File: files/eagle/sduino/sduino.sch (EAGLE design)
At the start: 13 parts, among them IC1 ATMEGA48/88/168-AU

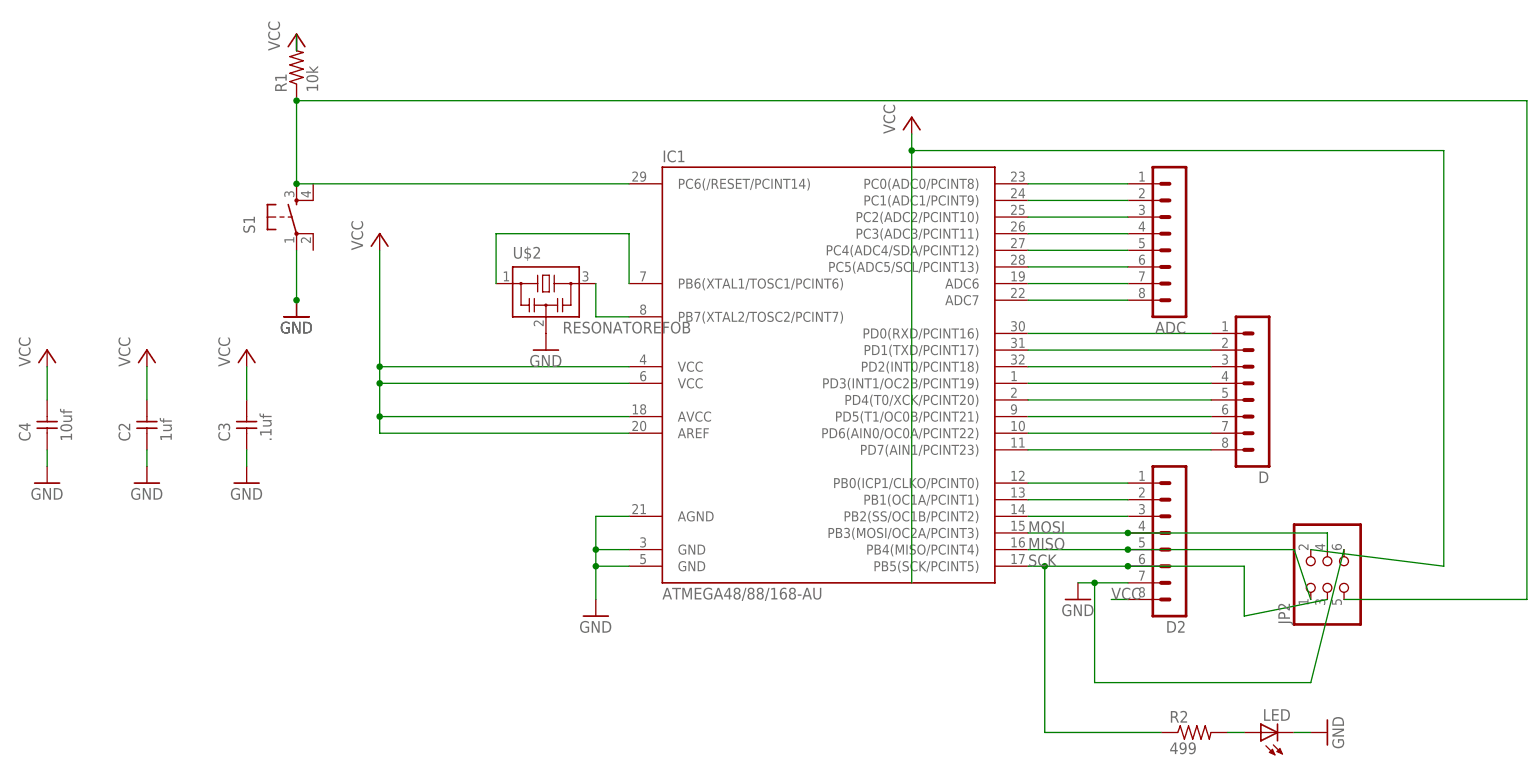
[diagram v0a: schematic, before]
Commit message: typo
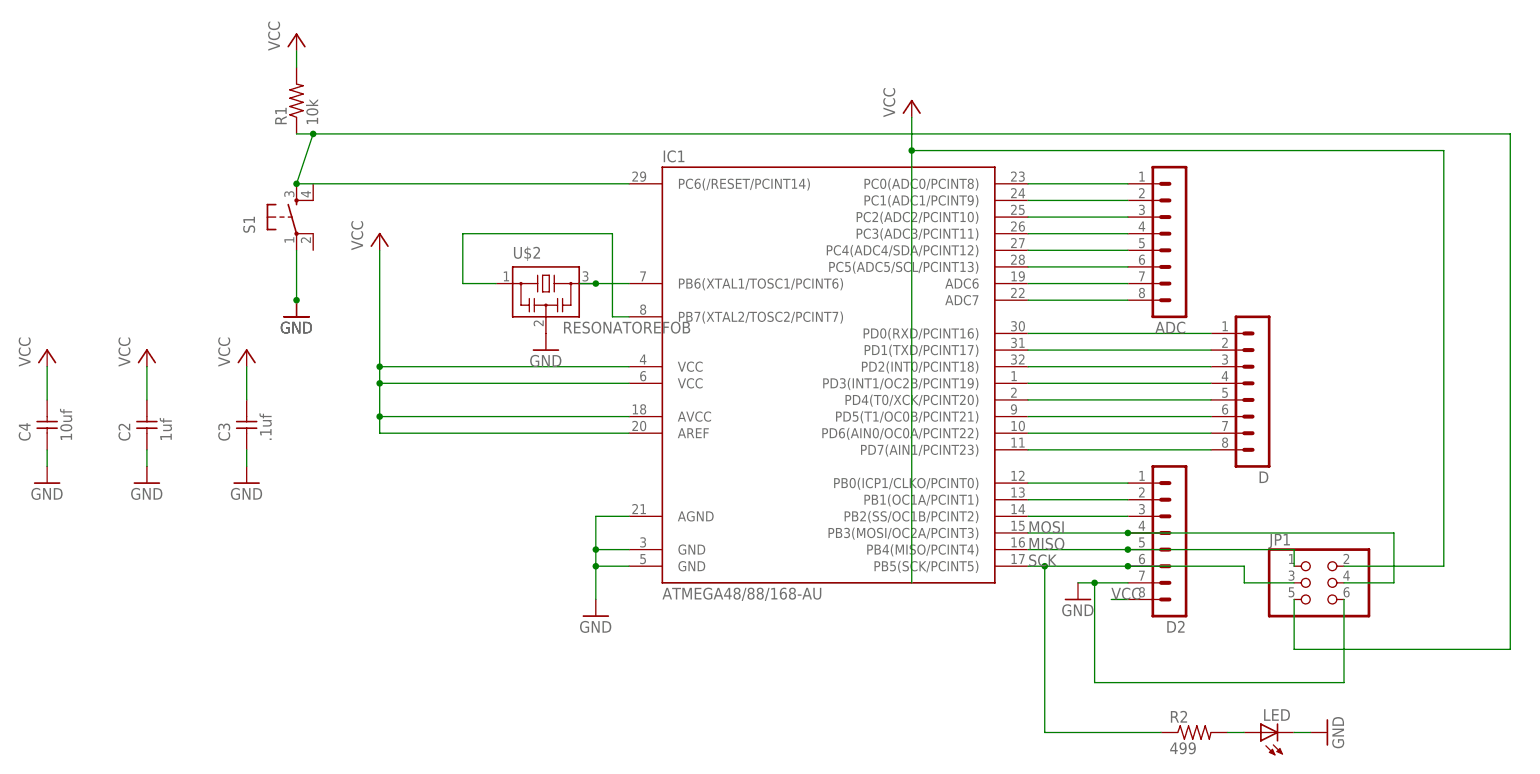
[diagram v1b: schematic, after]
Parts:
- removed JP2: (no value), fab:PINHD-2X3-SMD
- added JP1: (no value), pinhead:PINHD-2X3
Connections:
- removed net N$16: IC1.PB7(XTAL2/TOSC2/PCINT7), U$2.3
- new net N$9: IC1.PB6(XTAL1/TOSC1/PCINT6), U$2.3
- net GND: now also JP1.6; no longer JP2.6
- net MISO: now also JP1.1; no longer JP2.1
- net MOSI: now also JP1.4; no longer JP2.4
- net N$1: now also IC1.PB7(XTAL2/TOSC2/PCINT7); no longer IC1.PB6(XTAL1/TOSC1/PCINT6)
- net RST: now also JP1.5; no longer JP2.5
- net SCK: now also JP1.3; no longer JP2.3
- net VCC: now also JP1.2; no longer JP2.2
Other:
- moved on the sheet: R1
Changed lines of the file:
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@@
 <part name="U$2" library="fab" deviceset="RESONATOR" device="EFOB"/>
 <part name="GND10" library="supply1" deviceset="GND" device=""/>
-<part name="JP2" library="fab" deviceset="PINHD-2X3-SMD" device=""/>
+<part name="JP1" library="pinhead" deviceset="PINHD-2X3" device=""/>
 </parts>
 <sheets>
@@
 <instance part="GND1" gate="1" x="-40.64" y="58.42"/>
 <instance part="GND2" gate="1" x="5.08" y="12.7"/>
-<instance part="R1" gate="G$1" x="-40.64" y="96.52" rot="R90"/>
+<instance part="R1" gate="G$1" x="-40.64" y="91.44" rot="R90"/>
 <instance part="S1" gate="2" x="-40.64" y="73.66"/>
 <instance part="D" gate="1" x="106.68" y="48.26" rot="R180"/>
@@
 <instance part="C4" gate="1" x="-78.74" y="43.18" rot="R90"/>
 <instance part="ADC" gate="1" x="93.98" y="71.12" rot="R180"/>
-<instance part="P+3" gate="VCC" x="53.34" y="88.9"/>
+<instance part="P+3" gate="VCC" x="53.34" y="91.44"/>
 <instance part="D2" gate="1" x="93.98" y="25.4" rot="R180"/>
 <instance part="GND9" gate="1" x="78.74" y="15.24"/>
 <instance part="U$2" gate="G$1" x="-2.54" y="63.5"/>
 <instance part="GND10" gate="1" x="-2.54" y="53.34"/>
-<instance part="JP2" gate="A" x="116.84" y="17.78" rot="R90"/>
+<instance part="JP1" gate="A" x="114.3" y="17.78"/>
 </instances>
 <busses>
@@
 </segment>
 <segment>
-<wire x1="-40.64" y1="99.06" x2="-40.64" y2="101.6" width="0.1524" layer="91"/>
+<wire x1="-40.64" y1="99.06" x2="-40.64" y2="96.52" width="0.1524" layer="91"/>
 <pinref part="P+1" gate="VCC" pin="VCC"/>
 <pinref part="R1" gate="G$1" pin="2"/>
@@
 <wire x1="53.34" y1="17.78" x2="53.34" y2="83.82" width="0.1524" layer="91"/>
 <pinref part="P+3" gate="VCC" pin="VCC"/>
-<wire x1="53.34" y1="83.82" x2="53.34" y2="86.36" width="0.1524" layer="91"/>
+<wire x1="53.34" y1="83.82" x2="53.34" y2="88.9" width="0.1524" layer="91"/>
+<wire x1="134.62" y1="20.32" x2="119.38" y2="20.32" width="0.1524" layer="91"/>
 <wire x1="134.62" y1="20.32" x2="134.62" y2="83.82" width="0.1524" layer="91"/>
 <wire x1="134.62" y1="83.82" x2="53.34" y2="83.82" width="0.1524" layer="91"/>
 <junction x="53.34" y="83.82"/>
-<pinref part="JP2" gate="A" pin="2"/>
-<wire x1="134.62" y1="20.32" x2="114.3" y2="22.86" width="0.1524" layer="91"/>
+<pinref part="JP1" gate="A" pin="2"/>
 </segment>
 <segment>
@@
 <segment>
 <pinref part="R1" gate="G$1" pin="1"/>
-<wire x1="-40.64" y1="91.44" x2="147.32" y2="91.44" width="0.1524" layer="91"/>
-<wire x1="147.32" y1="91.44" x2="147.32" y2="15.24" width="0.1524" layer="91"/>
-<junction x="-40.64" y="91.44"/>
+<wire x1="-40.64" y1="86.36" x2="-38.1" y2="86.36" width="0.1524" layer="91"/>
+<wire x1="-38.1" y1="86.36" x2="144.78" y2="86.36" width="0.1524" layer="91"/>
+<wire x1="144.78" y1="86.36" x2="144.78" y2="7.62" width="0.1524" layer="91"/>
+<wire x1="144.78" y1="7.62" x2="111.76" y2="7.62" width="0.1524" layer="91"/>
+<wire x1="111.76" y1="7.62" x2="111.76" y2="15.24" width="0.1524" layer="91"/>
+<pinref part="JP1" gate="A" pin="5"/>
+<junction x="-38.1" y="86.36"/>
 <pinref part="S1" gate="2" pin="S"/>
-<wire x1="-40.64" y1="91.44" x2="-40.64" y2="78.74" width="0.1524" layer="91"/>
+<wire x1="-38.1" y1="86.36" x2="-40.64" y2="78.74" width="0.1524" layer="91"/>
 <pinref part="IC1" gate="1" pin="PC6(/RESET/PCINT14)"/>
 <wire x1="-40.64" y1="78.74" x2="10.16" y2="78.74" width="0.1524" layer="91"/>
 <junction x="-40.64" y="78.74"/>
-<pinref part="JP2" gate="A" pin="5"/>
-<wire x1="147.32" y1="15.24" x2="119.38" y2="15.24" width="0.1524" layer="91"/>
 </segment>
 </net>
@@
 <pinref part="GND9" gate="1" pin="GND"/>
 <wire x1="81.28" y1="17.78" x2="78.74" y2="17.78" width="0.1524" layer="91"/>
-<wire x1="114.3" y1="2.54" x2="81.28" y2="2.54" width="0.1524" layer="91"/>
+<wire x1="119.38" y1="15.24" x2="119.38" y2="2.54" width="0.1524" layer="91"/>
+<wire x1="119.38" y1="2.54" x2="81.28" y2="2.54" width="0.1524" layer="91"/>
 <wire x1="81.28" y1="2.54" x2="81.28" y2="17.78" width="0.1524" layer="91"/>
 <junction x="81.28" y="17.78"/>
-<pinref part="JP2" gate="A" pin="6"/>
-<wire x1="114.3" y1="2.54" x2="119.38" y2="22.86" width="0.1524" layer="91"/>
+<pinref part="JP1" gate="A" pin="6"/>
 </segment>
 </net>
@@
 <pinref part="IC1" gate="1" pin="PB3(MOSI/OC2A/PCINT3)"/>
 <pinref part="D2" gate="1" pin="4"/>
-<wire x1="86.36" y1="25.4" x2="116.84" y2="25.4" width="0.1524" layer="91"/>
+<wire x1="86.36" y1="25.4" x2="127" y2="25.4" width="0.1524" layer="91"/>
+<wire x1="127" y1="25.4" x2="127" y2="17.78" width="0.1524" layer="91"/>
 <junction x="86.36" y="25.4"/>
-<pinref part="JP2" gate="A" pin="4"/>
-<wire x1="116.84" y1="25.4" x2="116.84" y2="22.86" width="0.1524" layer="91"/>
+<wire x1="127" y1="17.78" x2="119.38" y2="17.78" width="0.1524" layer="91"/>
+<pinref part="JP1" gate="A" pin="4"/>
 </segment>
 </net>
@@
 <pinref part="D2" gate="1" pin="5"/>
 <wire x1="86.36" y1="22.86" x2="111.76" y2="22.86" width="0.1524" layer="91"/>
+<wire x1="111.76" y1="22.86" x2="111.76" y2="20.32" width="0.1524" layer="91"/>
 <junction x="86.36" y="22.86"/>
-<pinref part="JP2" gate="A" pin="1"/>
-<wire x1="111.76" y1="22.86" x2="114.3" y2="15.24" width="0.1524" layer="91"/>
+<pinref part="JP1" gate="A" pin="1"/>
 </segment>
 </net>
@@
 <pinref part="D2" gate="1" pin="6"/>
 <wire x1="86.36" y1="20.32" x2="104.14" y2="20.32" width="0.1524" layer="91"/>
-<wire x1="104.14" y1="20.32" x2="104.14" y2="12.7" width="0.1524" layer="91"/>
+<wire x1="104.14" y1="20.32" x2="104.14" y2="17.78" width="0.1524" layer="91"/>
 <junction x="86.36" y="20.32"/>
-<pinref part="JP2" gate="A" pin="3"/>
-<wire x1="104.14" y1="12.7" x2="116.84" y2="15.24" width="0.1524" layer="91"/>
+<wire x1="104.14" y1="17.78" x2="111.76" y2="17.78" width="0.1524" layer="91"/>
+<pinref part="JP1" gate="A" pin="3"/>
 </segment>
 </net>
@@
 </segment>
 </net>
+<net name="N$1" class="0">
+<segment>
+<wire x1="10.16" y1="58.42" x2="7.62" y2="58.42" width="0.1524" layer="91"/>
+<wire x1="7.62" y1="58.42" x2="7.62" y2="71.12" width="0.1524" layer="91"/>
+<wire x1="7.62" y1="71.12" x2="-15.24" y2="71.12" width="0.1524" layer="91"/>
+<wire x1="-15.24" y1="71.12" x2="-15.24" y2="63.5" width="0.1524" layer="91"/>
+<wire x1="-15.24" y1="63.5" x2="-10.16" y2="63.5" width="0.1524" layer="91"/>
+<pinref part="IC1" gate="1" pin="PB7(XTAL2/TOSC2/PCINT7)"/>
+<pinref part="U$2" gate="G$1" pin="1"/>
+</segment>
+</net>
+<net name="N$9" class="0">
+<segment>
+<wire x1="10.16" y1="63.5" x2="5.08" y2="63.5" width="0.1524" layer="91"/>
+<wire x1="5.08" y1="63.5" x2="2.54" y2="63.5" width="0.1524" layer="91"/>
+<junction x="5.08" y="63.5"/>
+<pinref part="IC1" gate="1" pin="PB6(XTAL1/TOSC1/PCINT6)"/>
+<pinref part="U$2" gate="G$1" pin="3"/>
+</segment>
+</net>
 <net name="N$10" class="0">
 <segment>
@@
 </segment>
 </net>
-<net name="N$16" class="0">
-<segment>
-<pinref part="IC1" gate="1" pin="PB7(XTAL2/TOSC2/PCINT7)"/>
-<pinref part="U$2" gate="G$1" pin="3"/>
-<wire x1="10.16" y1="58.42" x2="5.08" y2="58.42" width="0.1524" layer="91"/>
-<wire x1="5.08" y1="58.42" x2="5.08" y2="63.5" width="0.1524" layer="91"/>
-</segment>
-</net>
-<net name="N$1" class="0">
-<segment>
-<pinref part="IC1" gate="1" pin="PB6(XTAL1/TOSC1/PCINT6)"/>
-<wire x1="10.16" y1="63.5" x2="10.16" y2="71.12" width="0.1524" layer="91"/>
-<wire x1="10.16" y1="71.12" x2="-10.16" y2="71.12" width="0.1524" layer="91"/>
-<pinref part="U$2" gate="G$1" pin="1"/>
-<wire x1="-10.16" y1="71.12" x2="-10.16" y2="63.5" width="0.1524" layer="91"/>
-</segment>
-</net>
